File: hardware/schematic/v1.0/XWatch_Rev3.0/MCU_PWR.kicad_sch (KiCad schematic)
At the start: 32 parts, among them U1 STM32U5G9NJH6Q, U15 STM32U5A9BJY6QTR

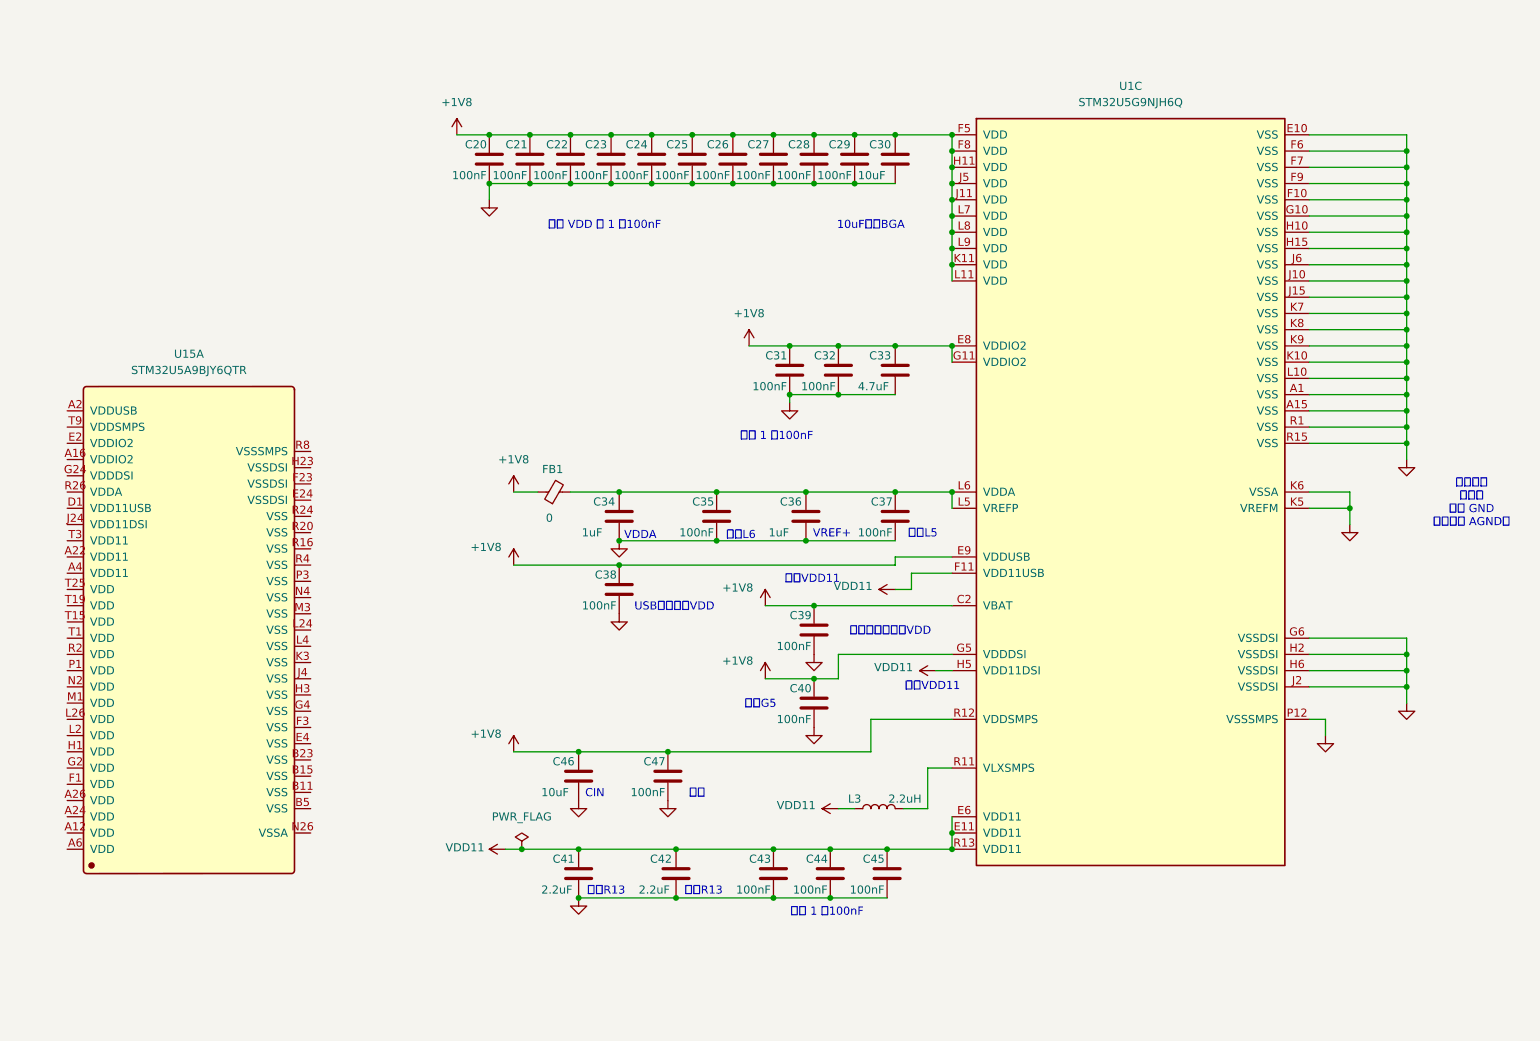
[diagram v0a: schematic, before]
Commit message: sch update
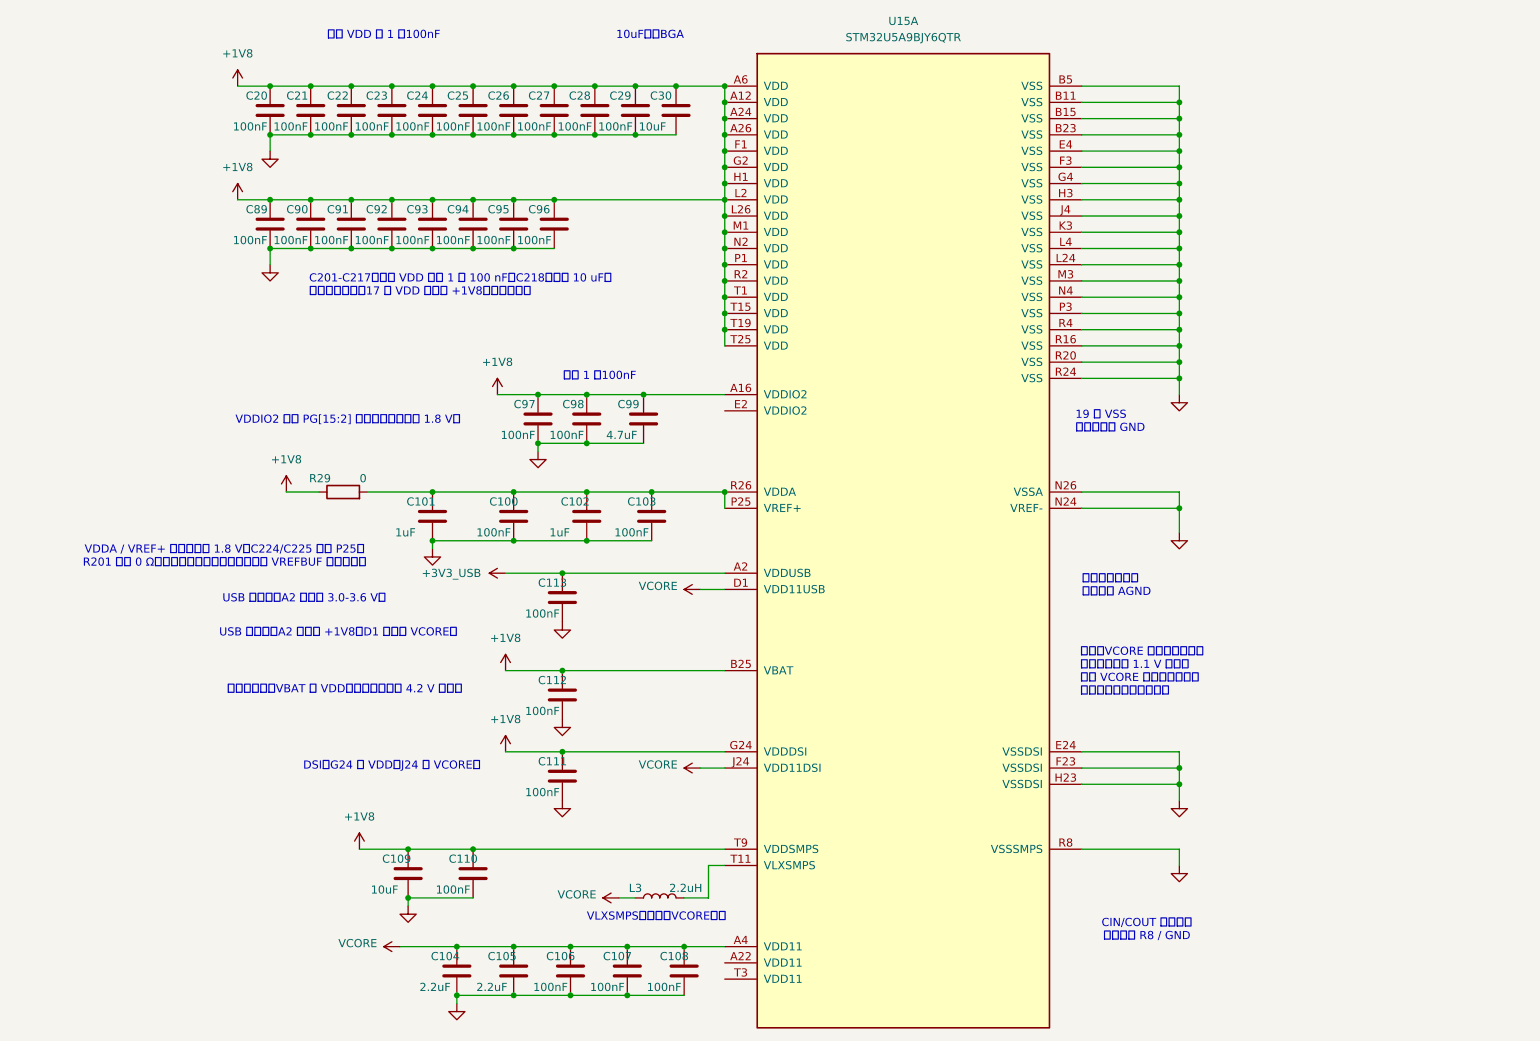
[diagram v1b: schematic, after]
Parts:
- removed C31, C32, C35, C37, C38, C39, C40, C43, C44, C45, C47: 100nF, XWatch_Rev3.0:GEN_C_0201, symbol XWatch_Rev3.0:C
- removed C33: 4.7uF, XWatch_Rev3.0:GEN_C_0402, symbol XWatch_Rev3.0:C
- removed C34, C36: 1uF, XWatch_Rev3.0:GEN_C_0402, symbol XWatch_Rev3.0:C
- removed C41, C42: 2.2uF, XWatch_Rev3.0:GEN_C_0402, symbol XWatch_Rev3.0:C
- removed C46: 10uF, XWatch_Rev3.0:GEN_C_0402, symbol XWatch_Rev3.0:C
- removed FB1: 0, symbol XWatch_Rev3.0:FerriteBead_Small
- removed U1: STM32U5G9NJH6Q, XWatch_Rev3.0:STM32U5G9NJH6Q, symbol XWatch_Rev3.0:STM32U5G9NJH6Q
- added C100, C103, C106, C107, C108, C110, C111, C112, C113, C89, C90, C91, C92, C93, C94, C95, C96, C97, C98: 100nF, XWatch_Rev3.0:GEN_C_0201, symbol XWatch_Rev3.0:C
- added C101, C102: 1uF, XWatch_Rev3.0:GEN_C_0402, symbol XWatch_Rev3.0:C
- added C104, C105: 2.2uF, XWatch_Rev3.0:GEN_C_0402, symbol XWatch_Rev3.0:C
- added C109: 10uF, XWatch_Rev3.0:GEN_C_0402, symbol XWatch_Rev3.0:C
- added C99: 4.7uF, XWatch_Rev3.0:GEN_C_0402, symbol XWatch_Rev3.0:C
- added R29: 0, XWatch_Rev3.0:GEN_R_0201, symbol XWatch_Rev3.0:R
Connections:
- net VDD11 is gone; now on net VCORE: L3.1
- net +1V8: now also U15.A12 (VDD), U15.A16 (VDDIO2), U15.A24 (VDD), U15.A26 (VDD), U15.A6 (VDD), U15.B25 (VBAT), U15.F1 (VDD), U15.G2 (VDD), U15.G24 (VDDDSI), U15.H1 (VDD), U15.L2 (VDD), U15.L26 (VDD), U15.M1 (VDD), U15.N2 (VDD), U15.P1 (VDD), U15.R2 (VDD), U15.T1 (VDD), U15.T15 (VDD), U15.T19 (VDD), U15.T25 (VDD), U15.T9 (VDDSMPS), C109.1, C110.1, C111.1, C112.1, C89.1, C90.1, C91.1, C92.1, C93.1, C94.1, C95.1, C96.1, C97.1, C98.1, C99.1, R29.1
- net GND: now also U15.B11 (VSS), U15.B15 (VSS), U15.B23 (VSS), U15.B5 (VSS), U15.E24 (VSSDSI), U15.E4 (VSS), U15.F23 (VSSDSI), U15.F3 (VSS), U15.G4 (VSS), U15.H23 (VSSDSI), U15.H3 (VSS), U15.J4 (VSS), U15.K3 (VSS), U15.L24 (VSS), U15.L4 (VSS), U15.M3 (VSS), U15.N24 (VREF-), U15.N26 (VSSA), U15.N4 (VSS), U15.P3 (VSS), U15.R16 (VSS), U15.R20 (VSS), U15.R24 (VSS), U15.R4 (VSS), U15.R8 (VSSSMPS), C100.2, C101.2, C102.2, C103.2, C104.2, C105.2, C106.2, C107.2, C108.2, C109.2, C110.2, C111.2, C112.2, C113.2, C89.2, C90.2, C91.2, C92.2, C93.2, C94.2, C95.2, C96.2, C97.2, C98.2, C99.2
- net at L3.2: now also U15.T11 (VLXSMPS)
- net +3V3_USB: now reaches U15.A2 (VDDUSB)
- net +3V3_USB: now also C113.1
- net VCORE: now reaches U15.A4 (VDD11)
- net VCORE: now also U15.D1 (VDD11USB), U15.J24 (VDD11DSI), C104.1, C105.1, C106.1, C107.1, C108.1
- net at U15.R26 (VDDA): now also U15.P25 (VREF+), C100.1, C101.1, C102.1, C103.1, R29.2
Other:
- note added: "19 个 VSS 全部接整板 GND"
- note added: "C201-C217：每个 VDD 球各 1 颗 100 nF；C218：整片 10 uF。 电容靠近球位；17 个 VDD 全部接 +1V8，不能遗漏。"
- note added: "CIN/COUT 接地回路 就近返回 R8 / GND"
- note added: "DSI：G24 同 VDD；J24 接 VCORE。"
- note added: "USB 不用时：A2 可改接 +1V8；D1 仍连接 VCORE。"
- note added: "USB 已启用：A2 必须为 3.0-3.6 V。"
- note added: "VDDA / VREF+ 同接滤波后 1.8 V；C224/C225 靠近 P25。 R201 默认 0 Ω；需要时经验证改为磁珠。内部 VREFBUF 保持关闭。"
- note added: "VDDIO2 控制 PG[15:2] 电平；本图统一为 1.8 V。"
- note added: "VLXSMPS引脚产生VCORE电压"
- note added: "同一完整地平面 不要割裂 AGND"
- note added: "无备用电池：VBAT 接 VDD；禁止直接满电 4.2 V 锂电。"
- note added: "注意：VCORE 是内部调压节点 不是固定外部 1.1 V 电源。 所有 VCORE 同名标签相连； 不用于给其他芯片供电。"
- note removed: "CIN"
- note removed: "USB不用，接VDD"
- note removed: "VDDA"
- note removed: "VREF+"
- note removed: "全部直接 打孔到 整层 GND （不分割 AGND）"
- note removed: "可选"
- note removed: "无备份电池，接VDD"
- note removed: "靠近G5"
- note removed: "靠近L5"
- note removed: "靠近L6"
- note removed: "靠近R13"
- note removed: "须接VDD11"
